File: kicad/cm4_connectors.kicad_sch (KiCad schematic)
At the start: 11 parts, among them J2 Header-Male-2.54_2x3, J3 Header-Male-2.54_1x3, J5 2541WV-2X12P, U15 74LVC1G07SE-7, U16 74LVC1G07SE-7

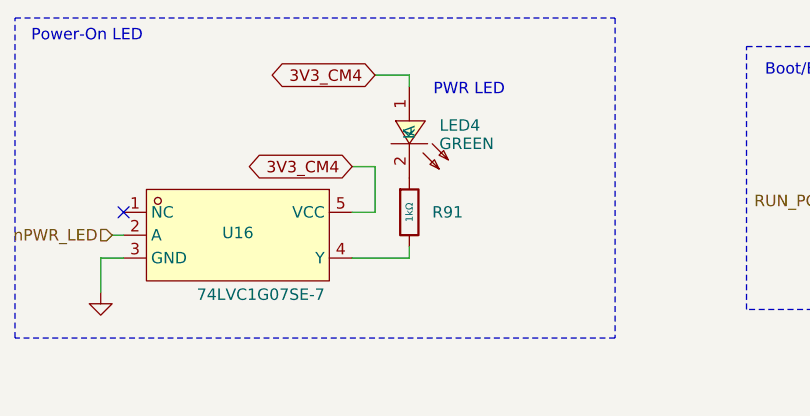
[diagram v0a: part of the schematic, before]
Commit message: Before removing CAN 24V
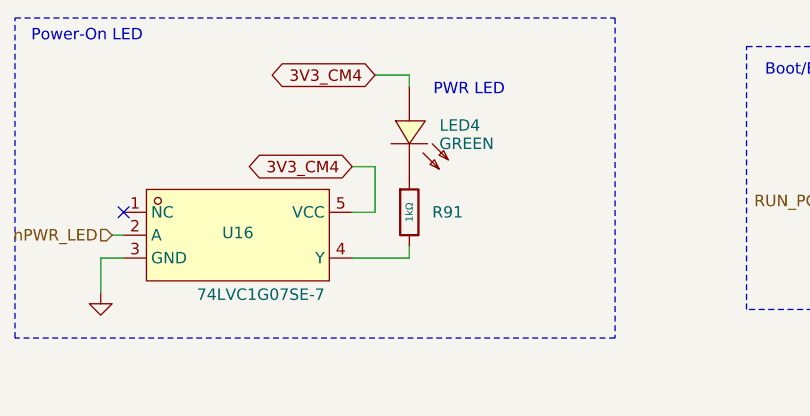
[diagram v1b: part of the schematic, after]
